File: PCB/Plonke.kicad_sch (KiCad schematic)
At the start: 17 parts, among them J1 USB_C_Receptacle_USB2.0_16P, J2 AVR-ISP-6, U1 ATmega32U4-A, U2 USB6B1, Y1 Crystal_GND24_Small

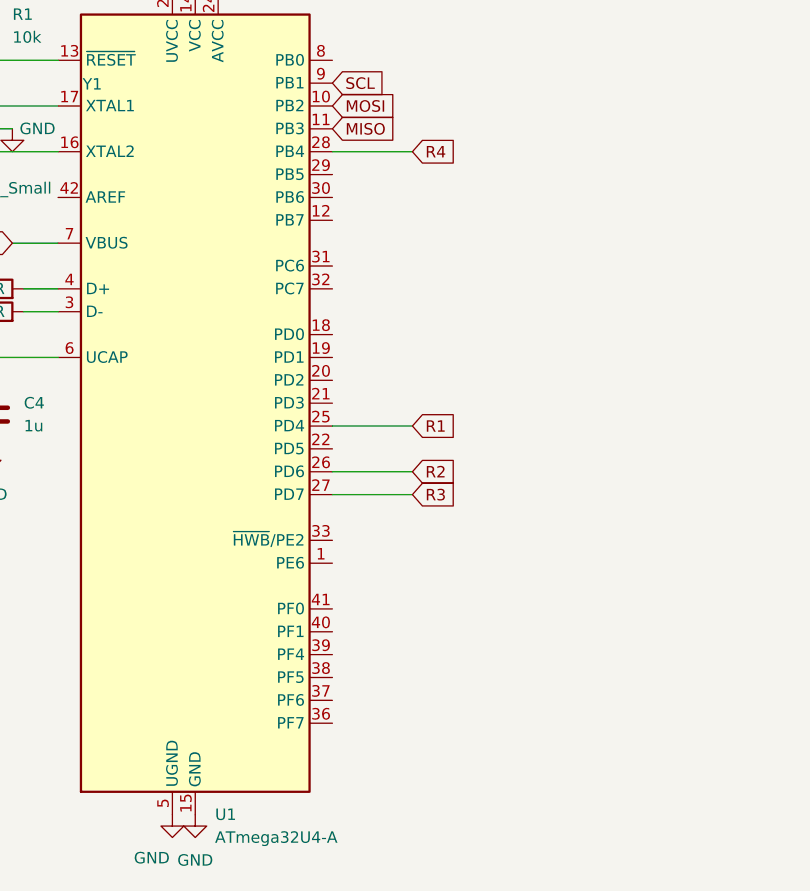
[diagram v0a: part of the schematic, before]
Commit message: WIRING DONE
lfg
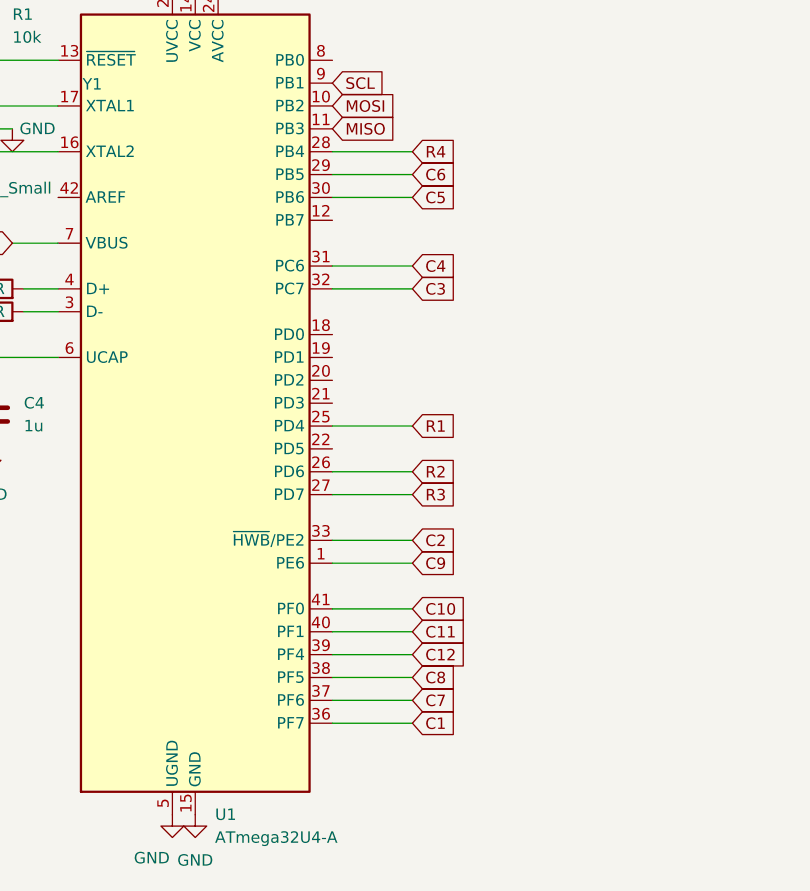
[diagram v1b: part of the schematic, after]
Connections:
- net C9: now reaches U1.1 (PE6)
- net C6: now reaches U1.29 (PB5)
- net C5: now reaches U1.30 (PB6)
- net C4: now reaches U1.31 (PC6)
- net C3: now reaches U1.32 (PC7)
- net C2: now reaches U1.33 (~{HWB}/PE2)
- net C1: now reaches U1.36 (PF7)
- net C7: now reaches U1.37 (PF6)
- net C8: now reaches U1.38 (PF5)
- net C12: now reaches U1.39 (PF4)
- net C11: now reaches U1.40 (PF1)
- net C10: now reaches U1.41 (PF0)
